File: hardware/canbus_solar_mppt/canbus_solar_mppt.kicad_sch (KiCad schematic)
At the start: 27 parts

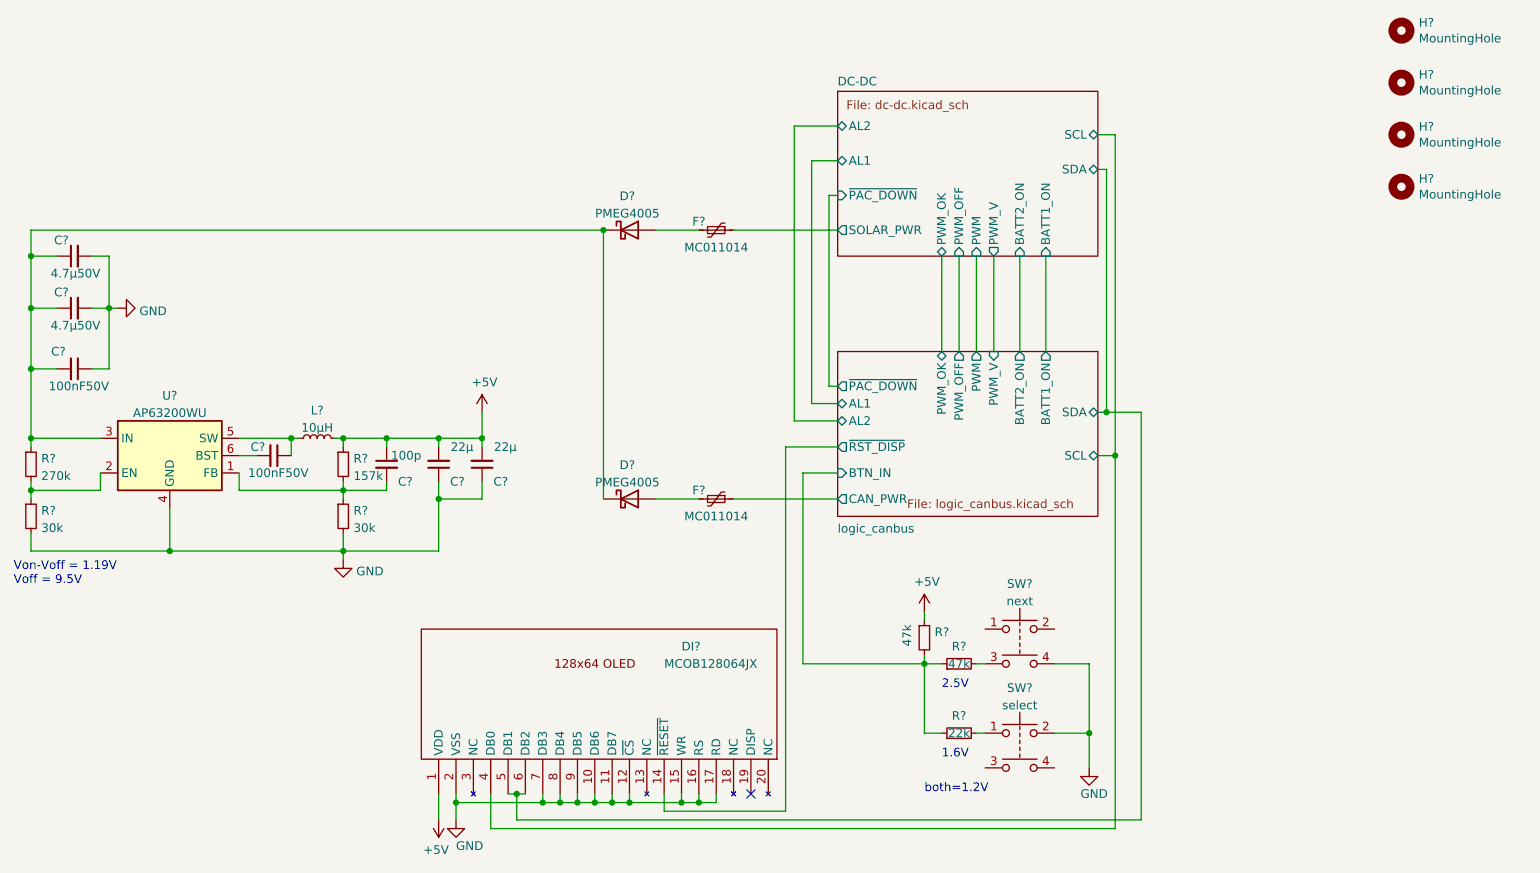
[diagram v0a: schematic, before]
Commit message: Add footprint for OLED display annotate schematic run and fix ERC
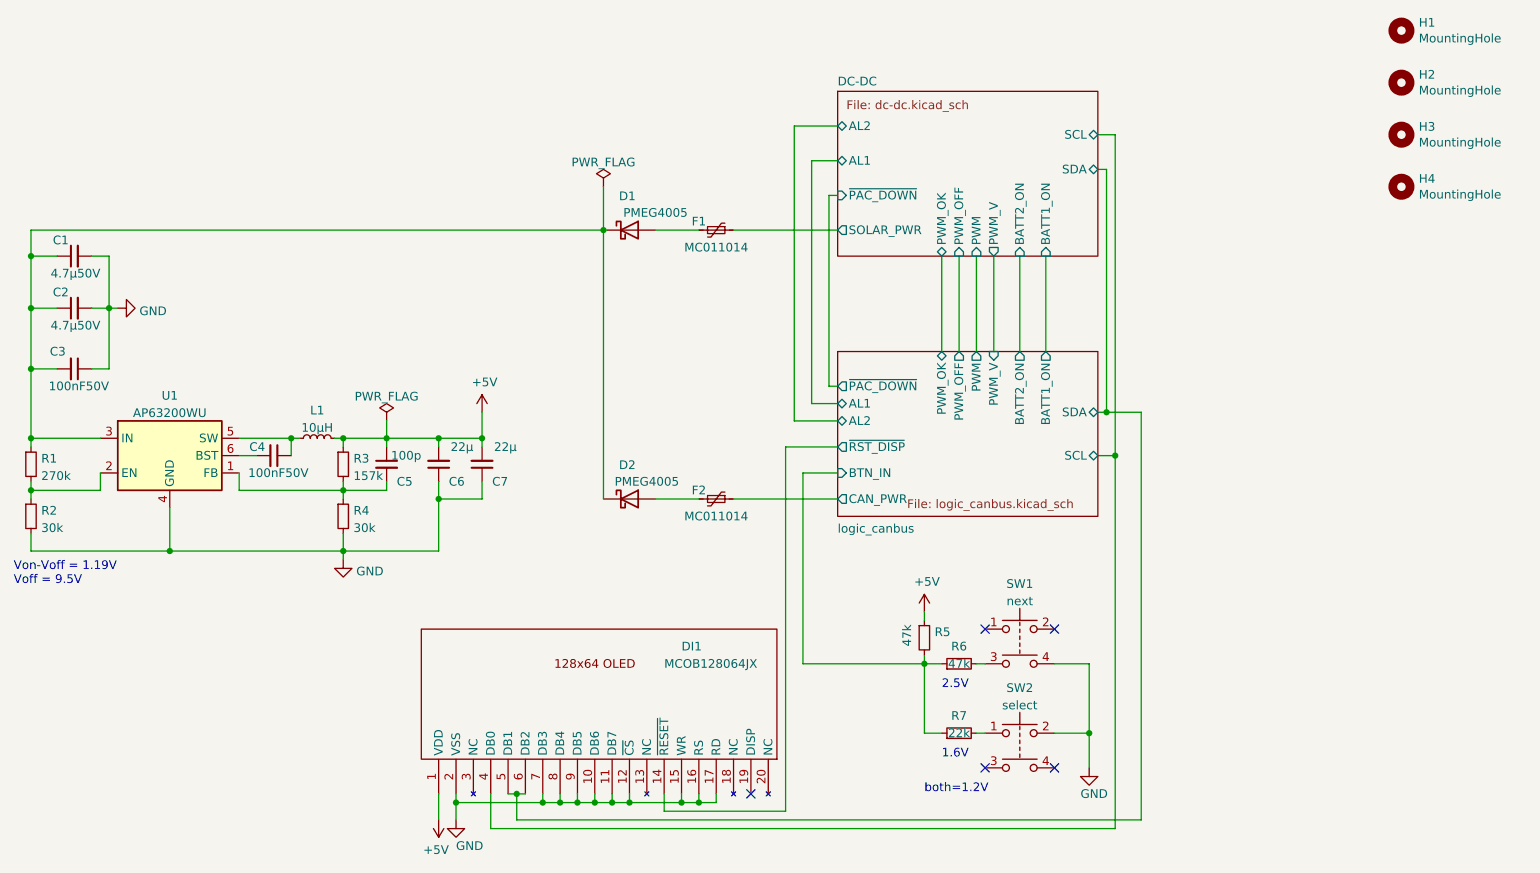
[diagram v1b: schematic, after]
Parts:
- DI1: renamed from DI?; footprint (none) -> LCDdisplays.mod:MCOB128064JX; P/N (none) -> MCOB128064JX-YM
- gave numbers to parts that had none: 26
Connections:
- no-connect marks 1 -> 5
